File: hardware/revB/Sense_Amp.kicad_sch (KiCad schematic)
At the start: 4 parts, among them U13 INA240A3EDRQ1

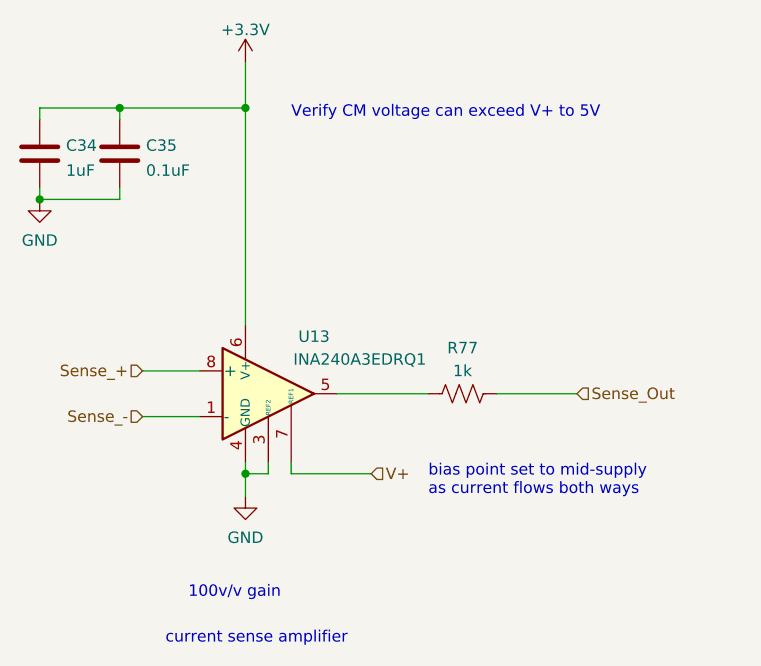
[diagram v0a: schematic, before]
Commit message: working
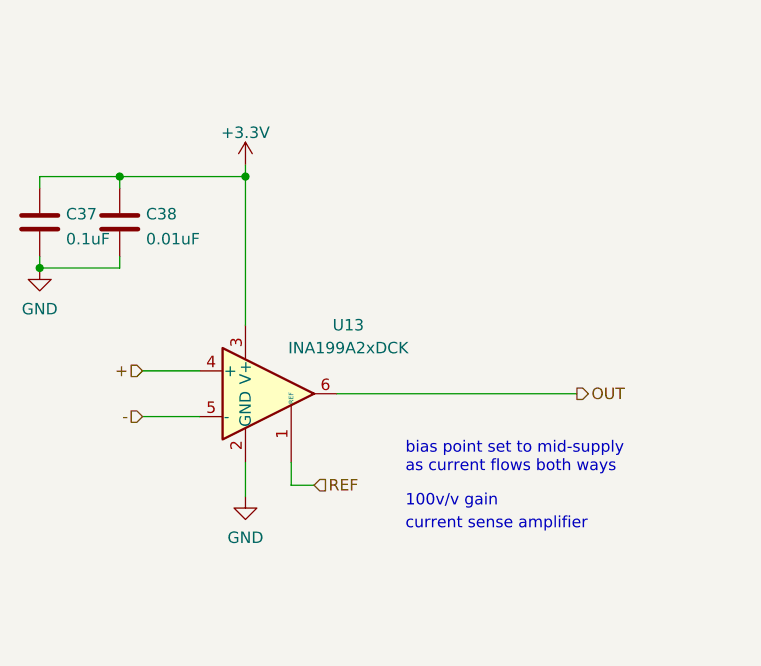
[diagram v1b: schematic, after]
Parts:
- removed R77: 1k, Resistor_SMD:R_0603_1608Metric, symbol Device:R_US
- removed U13: INA240A3EDRQ1, Package_SO:SOIC-8_3.9x4.9mm_P1.27mm, symbol FP-Interface-Card:INA240AxxD
- added U13: INA199A2xDCK, Package_TO_SOT_SMD:SOT-363_SC-70-6, symbol Amplifier_Current:INA199xxDCK
- C37: renamed from C34; value 1uF -> 0.1uF
- C38: renamed from C35; value 0.1uF -> 0.01uF
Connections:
- net +3.3V: now also U13.3 (V+)
- net GND: now also U13.2 (GND)
- new net +: U13.4 (+)
- new net -: U13.5 (-)
- new net OUT: U13.6
- new net REF: U13.1 (REF)
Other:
- note removed: "Verify CM voltage can exceed V+ to 5V"
- company: Sierra Lobo INC -> (none)
- title: (none) -> Foras Promineo Payload Interface Board
- moved on the sheet: C37, C38
